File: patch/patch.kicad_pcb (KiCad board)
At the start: 2 copper layers, 26.5 x 16.5 mm, 20 parts, among them IC1 LTC3261, J1 -5V, J2 5V, J3 GND, J4 Audio_IN, J5 S_B, J6 SAW, J7 S_A, U1 AD8611

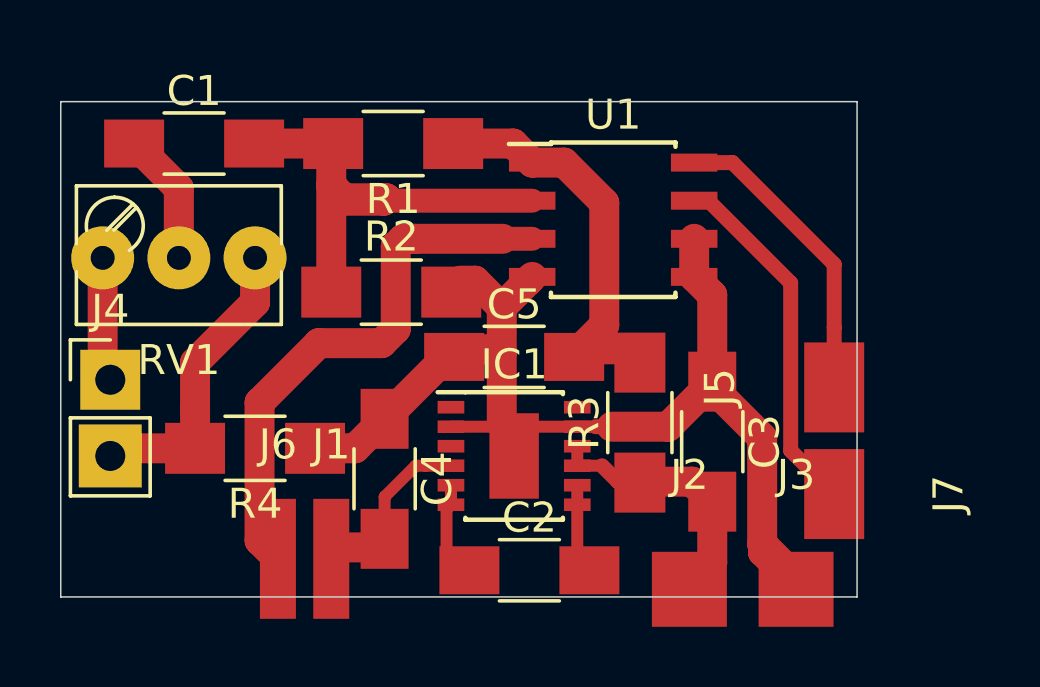
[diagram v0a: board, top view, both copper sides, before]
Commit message: p2
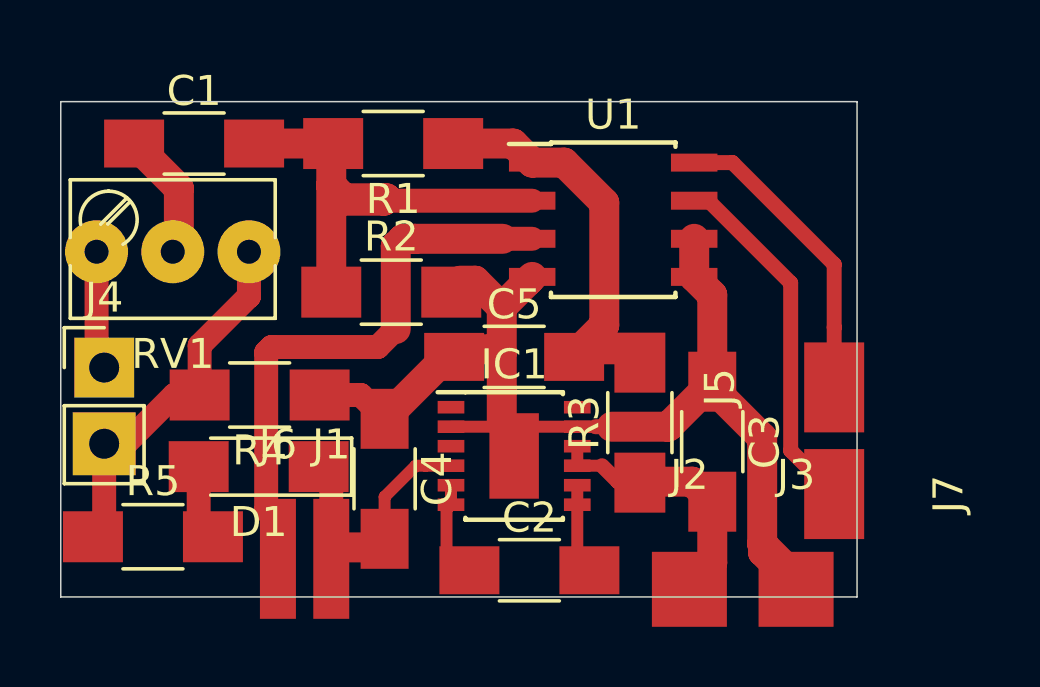
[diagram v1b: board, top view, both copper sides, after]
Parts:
- added D1: LED, LEDs:LED_1206_HandSoldering, F.Cu at (174.4, 116.9)
- added R5: 2k2, Resistors_SMD:R_1206_HandSoldering, F.Cu at (170.8, 119.3)
- moved R4 1.78 mm to (174.4, 114.6)
- moved J4 0.45 mm to (169.2, 113.6)
- moved RV1 0.29 mm to (169.0, 109.8)
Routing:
- net -5V: track 5.94 -> 9.19 mm
- net Net-(D1-Pad2): track 0.00 -> 2.53 mm
- net GND: track 62.1 -> 64.3 mm
- net Net-(J6-Pad1): track 18.4 -> 19.1 mm
